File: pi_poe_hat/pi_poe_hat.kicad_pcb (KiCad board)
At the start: 2 copper layers, 65.1 x 30.1 mm, 54 parts, among them J1 8P8C_LED_Shielded, T1 POE13P-50LD, U2 MP8007GV-Z, U4 RTL8152B, Y1 25MHz

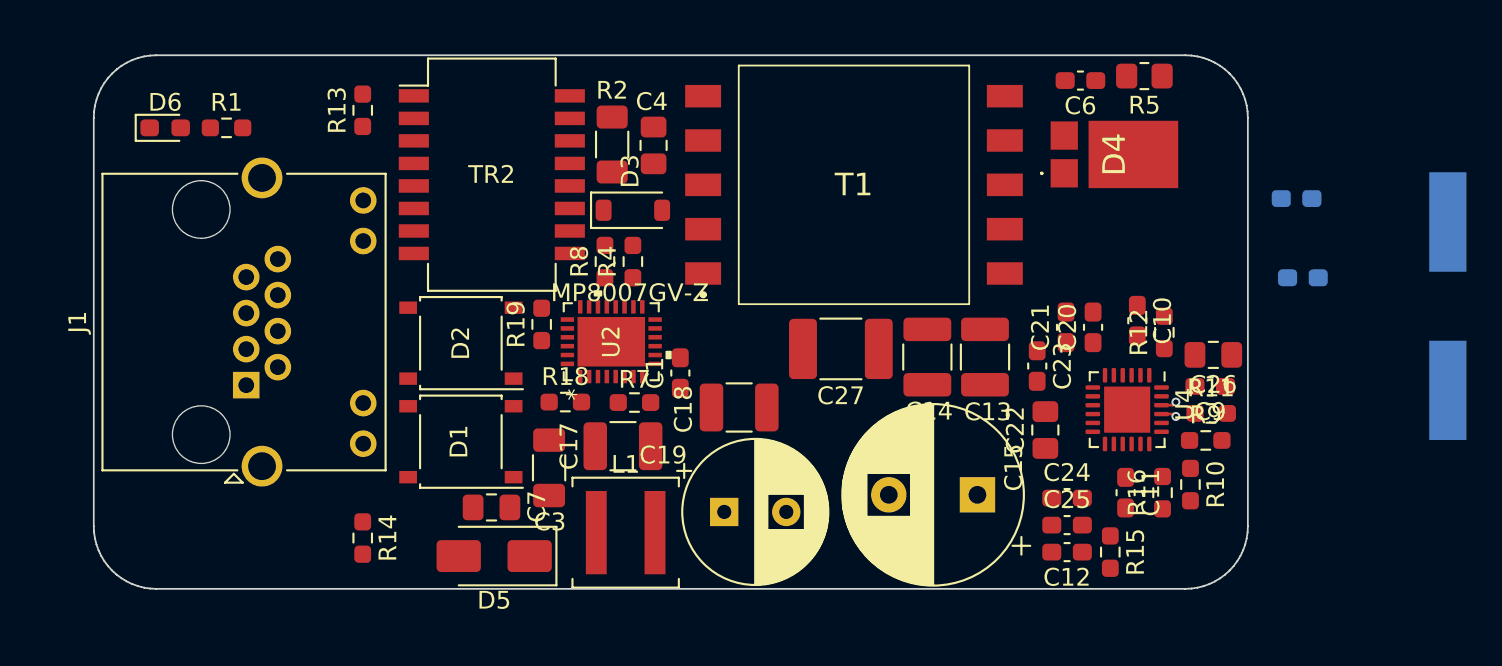
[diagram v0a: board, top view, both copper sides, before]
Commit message: v 1.0 of pcb almost done
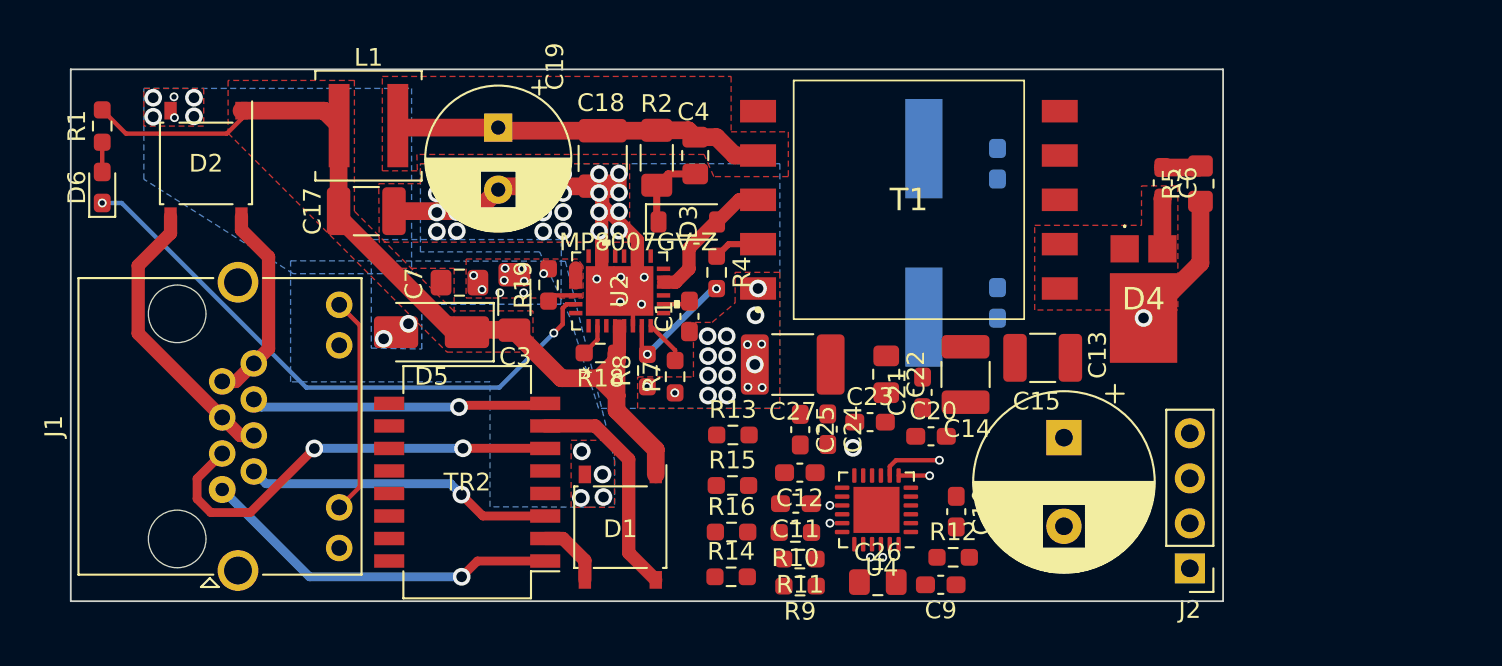
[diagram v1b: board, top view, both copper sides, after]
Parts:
- added J2: Conn_01x04, Connector_PinHeader_2.54mm:PinHeader_1x04_P2.54mm_Vertical, F.Cu at (136.7, 128.1)
- moved Y1 29.8 mm to (121.7, 109.1)
- moved R13 27.8 mm to (111.0, 120.5), turned to 0 degrees
- moved L1 27.2 mm to (90.4, 103.1)
- moved C19 25.2 mm to (97.7, 103.2), turned to -90 degrees
- moved R11 24.6 mm to (114.7, 127.5), turned to 180 degrees
- moved R16 24.4 mm to (110.9, 126.0), turned to 0 degrees
- moved R9 24.3 mm to (114.7, 129.1), turned to 180 degrees
- moved C26 22.9 mm to (119.1, 128.8), turned to 0 degrees
- moved R10 22.4 mm to (114.5, 126.0), turned to 180 degrees
- moved R15 21.6 mm to (110.9, 123.4), turned to 0 degrees
- moved R14 20.9 mm to (110.8, 128.5), turned to 0 degrees
- moved C17 19.6 mm to (90.3, 107.9)
- moved C9 18.9 mm to (122.7, 129.0)
- moved C11 18.6 mm to (114.5, 124.4), turned to 180 degrees
- moved C8 18.4 mm to (125.9, 105.2), turned to -90 degrees
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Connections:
- J1 pad 4: PoE+_2 -> PoE-_2
- J1 pad 5: PoE+_2 -> PoE-_2
- J1 pad 7: PoE-_2 -> PoE+_2
- J1 pad 8: PoE-_2 -> PoE+_2
- T1 pad 10: GND -> Net-(D4-A_1)
- T1 pad 7: Net-(D4-A_1) -> GND
- T1 pad 8: Net-(D4-A_1) -> GND
- T1 pad 9: GND -> Net-(D4-A_1)
- TR2 pad 2: PoE+_1 -> PoE-_1
- TR2 pad 7: PoE-_1 -> PoE+_1
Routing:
- net VDD: track 0.00 -> 51.3 mm
- net Net-(D6-K): track 0.00 -> 33.5 mm, vias 0 -> 2
- net GNDD: track 0.00 -> 32.2 mm, vias 0 -> 46
- net Net-(TR2-RD+): track 0.00 -> 24.6 mm, vias 0 -> 2
- net TRANS: track 0.00 -> 21.0 mm
- net Net-(TR2-TD+): track 0.00 -> 20.6 mm, vias 0 -> 1
- net Net-(TR2-TD-): track 0.00 -> 17.5 mm, vias 0 -> 1
- net Net-(TR2-RD-): track 0.00 -> 16.7 mm, vias 0 -> 1
- net PoE-_2: track 0.00 -> 16.3 mm
- net PoE+_1: track 0.00 -> 12.9 mm
- net /VDD33: track 0.00 -> 12.4 mm
- net PoE+_2: track 0.00 -> 11.5 mm
- net +5V: track 0.00 -> 7.97 mm, vias 0 -> 2
- net /SW: track 0.00 -> 7.93 mm
- net /FB1: track 0.00 -> 7.18 mm, vias 0 -> 2
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- added copper zone on B.Cu, net GNDD
- added copper zone on F.Cu, net GNDD
- added copper zone on F.Cu, net Net-(D4-A_1)
- added copper zone on F.Cu, net TRANS
- added copper zone on F.Cu, net VDD
- added copper zone on B.Cu, net VSS
- added copper zone on F.Cu, net VSS
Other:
- board size 65.1 x 30.1 mm -> 65 x 30 mm
